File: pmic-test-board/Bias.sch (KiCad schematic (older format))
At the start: 19 parts, among them J301 Conn_Coaxial, J302 Conn_02x04_Odd_Even, U301 AZ431LANTR-G1, U302 DS4424N+

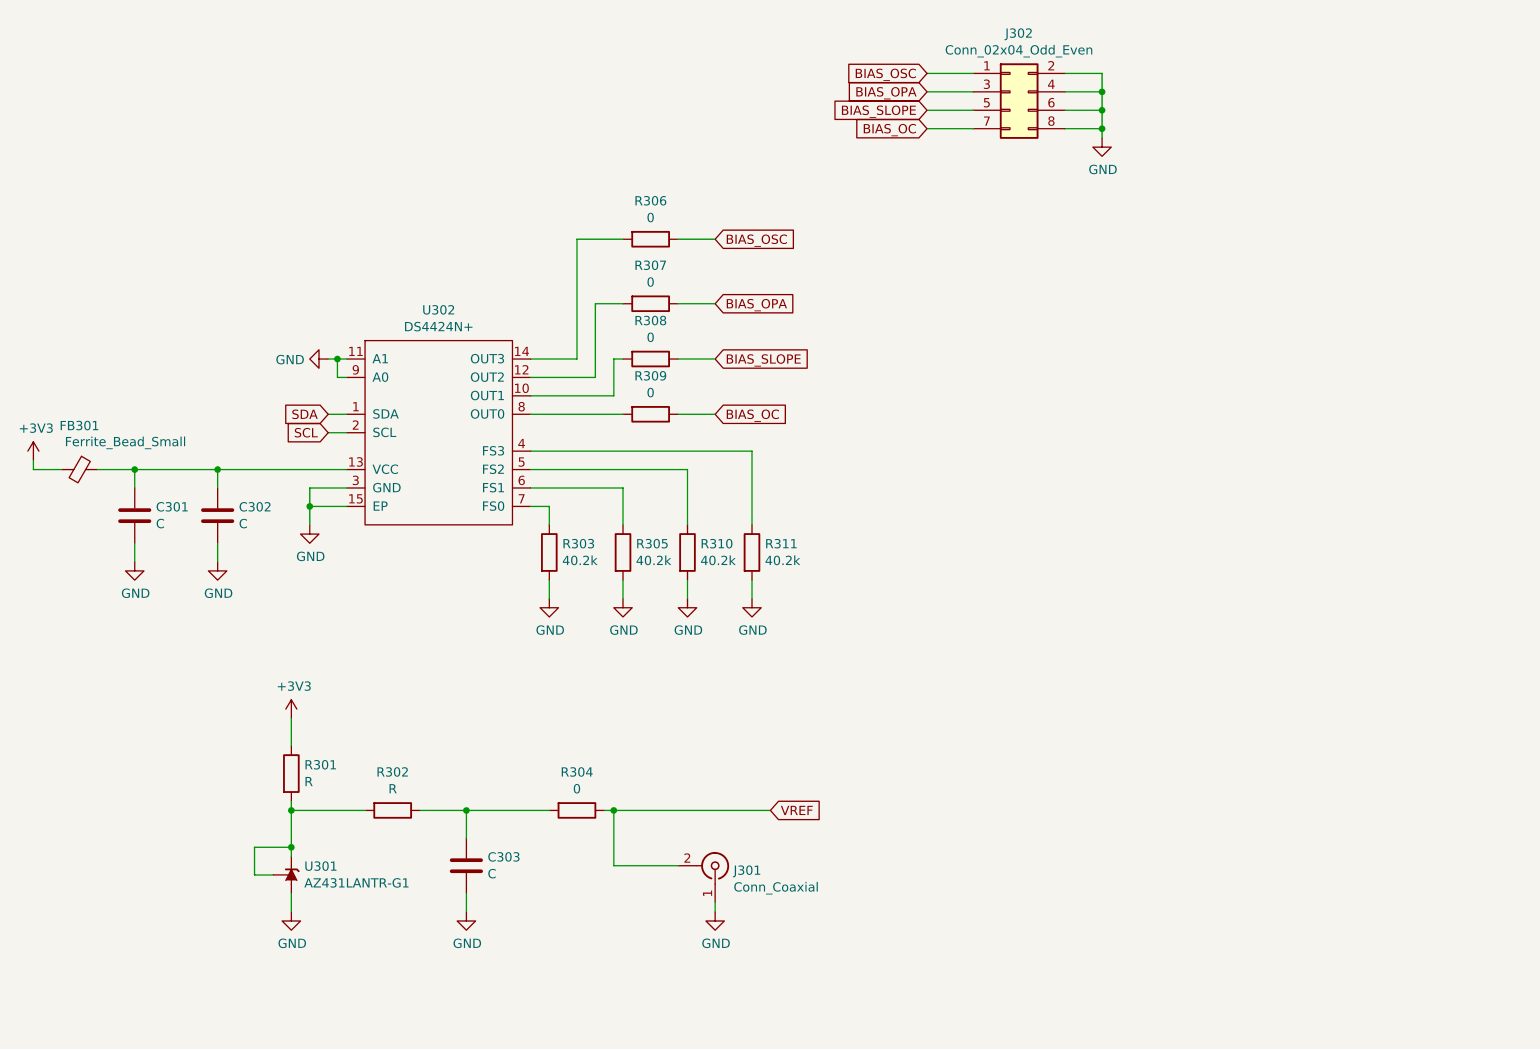
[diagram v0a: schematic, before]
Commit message: PCB routing done
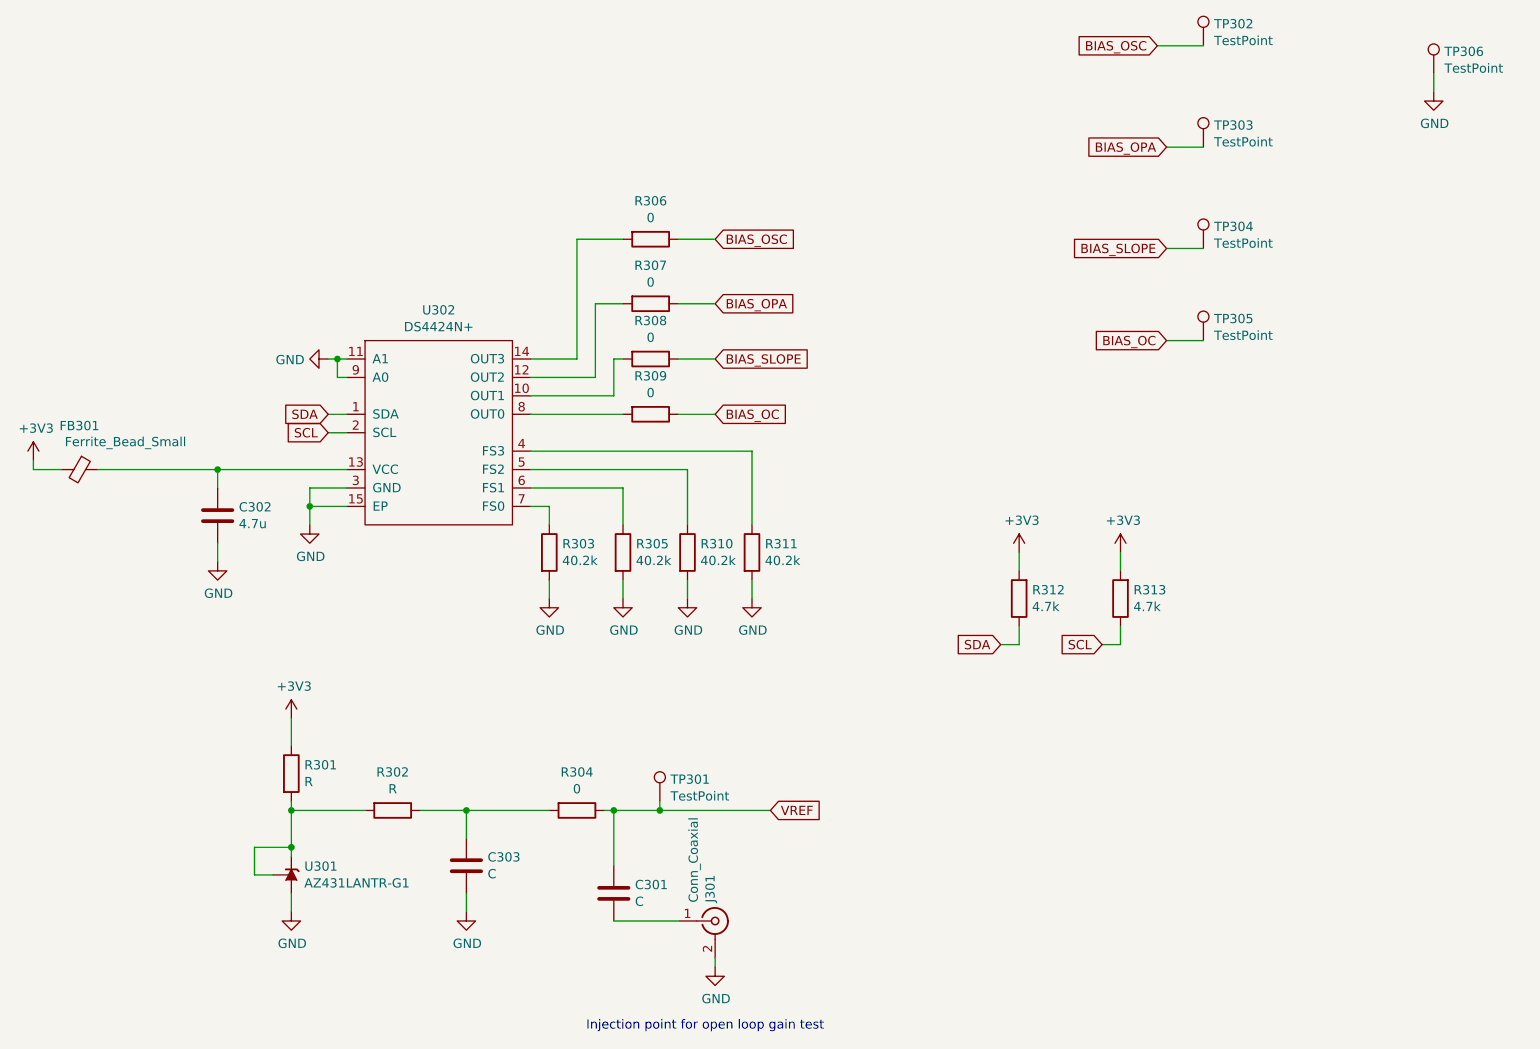
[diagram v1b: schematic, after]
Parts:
- removed J302: Conn_02x04_Odd_Even, symbol Connector_Generic:Conn_02x04_Odd_Even
- added R312, R313: 4.7k, Resistor_SMD:R_0603_1608Metric, symbol Device:R
- added TP301, TP302, TP303, TP304, TP305, TP306: TestPoint, wbraun_smd:THM_COMPACT, symbol Connector:TestPoint
- C302: value C -> 4.7u
- J301: footprint (none) -> Connector_Coaxial:SMA_Amphenol_132134_Vertical
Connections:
- net +3V3: now also R312.2, R313.2
- net BIAS_OC: now also TP305.1
- net BIAS_OPA: now also TP303.1
- net BIAS_OSC: now also TP302.1
- net BIAS_SLOPE: now also TP304.1
- net GND: now also J301.2 (Ext), TP306.1; no longer C301.2, J301.1 (In)
- net SCL: now also R313.1
- net SDA: now also R312.1
- net VREF: now also C301.1, TP301.1; no longer J301.2 (Ext)
- net at C302.1, FB301.1, U302.13 (VCC): no longer C301.1
- new net: C301.2, J301.1 (In)
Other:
- note added: "Injection point for open loop gain test"
- moved on the sheet: J301
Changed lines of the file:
@@
-$EndComp
-$Comp
-L Device:C C301
-U 1 1 619C3183
-P 1750 4100
-F 0 "C301" H 1865 4146 50  0000 L CNN
-F 1 "C" H 1865 4055 50  0000 L CNN
-F 2 "Capacitor_SMD:C_0603_1608Metric" H 1788 3950 50  0001 C CNN
-F 3 "~" H 1750 4100 50  0001 C CNN
-	1    1750 4100
-	1    0    0    -1
 $EndComp
 $Comp
@@
 P 2200 4100
 F 0 "C302" H 2315 4146 50  0000 L CNN
-F 1 "C" H 2315 4055 50  0000 L CNN
+F 1 "4.7u" H 2315 4055 50  0000 L CNN
 F 2 "Capacitor_SMD:C_0603_1608Metric" H 2238 3950 50  0001 C CNN
 F 3 "~" H 2200 4100 50  0001 C CNN
@@
 Wire Wire Line
 	2200 3950 2200 3850
-Wire Wire Line
-	1750 3950 1750 3850
-Wire Wire Line
-	1750 3850 2200 3850
-$Comp
-L power:GND #PWR0175
-U 1 1 619C47B0
-P 1750 4350
-F 0 "#PWR0175" H 1750 4100 50  0001 C CNN
-F 1 "GND" H 1755 4177 50  0000 C CNN
-F 2 "" H 1750 4350 50  0001 C CNN
-F 3 "" H 1750 4350 50  0001 C CNN
-	1    1750 4350
-	1    0    0    -1
-$EndComp
-Wire Wire Line
-	1750 4250 1750 4350
-Wire Wire Line
-	1550 3850 1750 3850
-Connection ~ 1750 3850
 Wire Wire Line
 	1350 3850 1200 3850
@@
 L Connector:Conn_Coaxial J301
 U 1 1 61A263C9
-P 4900 6000
-F 0 "J301" V 4874 6100 50  0000 L CNN
-F 1 "Conn_Coaxial" V 4783 6100 50  0000 L CNN
-F 2 "" H 4900 6000 50  0001 C CNN
-F 3 " ~" H 4900 6000 50  0001 C CNN
-	1    4900 6000
-	0    1    -1   0
+P 4900 6300
+F 0 "J301" V 4874 6400 50  0000 L CNN
+F 1 "Conn_Coaxial" V 4783 6400 50  0000 L CNN
+F 2 "Connector_Coaxial:SMA_Amphenol_132134_Vertical" H 4900 6300 50  0001 C CNN
+F 3 " ~" H 4900 6300 50  0001 C CNN
+	1    4900 6300
+	1    0    0    -1
 $EndComp
 $Comp
 L power:GND #PWR0185
 U 1 1 61A27901
-P 4900 6250
-F 0 "#PWR0185" H 4900 6000 50  0001 C CNN
-F 1 "GND" H 4905 6077 50  0000 C CNN
-F 2 "" H 4900 6250 50  0001 C CNN
-F 3 "" H 4900 6250 50  0001 C CNN
-	1    4900 6250
-	1    0    0    -1
-$EndComp
-Wire Wire Line
-	4900 6250 4900 6200
+P 4900 6550
+F 0 "#PWR0185" H 4900 6300 50  0001 C CNN
+F 1 "GND" H 4905 6377 50  0000 C CNN
+F 2 "" H 4900 6550 50  0001 C CNN
+F 3 "" H 4900 6550 50  0001 C CNN
+	1    4900 6550
+	1    0    0    -1
+$EndComp
+Wire Wire Line
+	4900 6550 4900 6500
 $Comp
 L Device:R R304
@@
 $EndComp
 Wire Wire Line
-	4700 6000 4350 6000
+	4700 6300 4350 6300
 Wire Wire Line
 	4350 6000 4350 5700
@@
 	4350 5700 4300 5700
 Wire Wire Line
-	4350 5700 5200 5700
+	4350 5700 4600 5700
 Connection ~ 4350 5700
 Text GLabel 5200 5700 2    50   Input ~ 0
 VREF
-$Comp
-L Connector_Generic:Conn_02x04_Odd_Even J302
-U 1 1 61A2AA7E
-P 6500 1800
-F 0 "J302" H 6550 2117 50  0000 C CNN
-F 1 "Conn_02x04_Odd_Even" H 6550 2026 50  0000 C CNN
-F 2 "" H 6500 1800 50  0001 C CNN
-F 3 "~" H 6500 1800 50  0001 C CNN
-	1    6500 1800
-	1    0    0    -1
-$EndComp
 $Comp
 L Device:R R306
@@
 Text GLabel 4900 3550 2    50   Input ~ 0
 BIAS_OC
-$Comp
-L power:GND #PWR0186
-U 1 1 61A39A05
-P 7000 2050
-F 0 "#PWR0186" H 7000 1800 50  0001 C CNN
-F 1 "GND" H 7005 1877 50  0000 C CNN
-F 2 "" H 7000 2050 50  0001 C CNN
-F 3 "" H 7000 2050 50  0001 C CNN
-	1    7000 2050
-	1    0    0    -1
-$EndComp
-Text GLabel 6050 1700 0    50   Input ~ 0
+Text GLabel 7300 1550 0    50   Input ~ 0
 BIAS_OSC
-Text GLabel 6050 1800 0    50   Input ~ 0
+Text GLabel 7350 2100 0    50   Input ~ 0
 BIAS_OPA
-Text GLabel 6050 1900 0    50   Input ~ 0
+Text GLabel 7350 2650 0    50   Input ~ 0
 BIAS_SLOPE
-Text GLabel 6050 2000 0    50   Input ~ 0
+Text GLabel 7350 3150 0    50   Input ~ 0
 BIAS_OC
-Wire Wire Line
-	6300 1700 6050 1700
-Wire Wire Line
-	6300 1800 6050 1800
-Wire Wire Line
-	6300 1900 6050 1900
-Wire Wire Line
-	6300 2000 6050 2000
-Wire Wire Line
-	6800 1700 7000 1700
-Wire Wire Line
-	7000 1700 7000 1800
-Wire Wire Line
-	6800 1800 7000 1800
-Connection ~ 7000 1800
-Wire Wire Line
-	7000 1800 7000 1900
-Wire Wire Line
-	6800 1900 7000 1900
-Connection ~ 7000 1900
-Wire Wire Line
-	7000 1900 7000 2000
-Wire Wire Line
-	6800 2000 7000 2000
-Connection ~ 7000 2000
-Wire Wire Line
-	7000 2000 7000 2050
+$Comp
+L Connector:TestPoint TP302
+U 1 1 6219CA5D
+P 7550 1550
+F 0 "TP302" H 7608 1668 50  0000 L CNN
+F 1 "TestPoint" H 7608 1577 50  0000 L CNN
+F 2 "wbraun_smd:THM_COMPACT" H 7750 1550 50  0001 C CNN
+F 3 "~" H 7750 1550 50  0001 C CNN
+	1    7550 1550
+	1    0    0    -1
+$EndComp
+$Comp
+L Connector:TestPoint TP303
+U 1 1 6219E164
+P 7550 2100
+F 0 "TP303" H 7608 2218 50  0000 L CNN
+F 1 "TestPoint" H 7608 2127 50  0000 L CNN
+F 2 "wbraun_smd:THM_COMPACT" H 7750 2100 50  0001 C CNN
+F 3 "~" H 7750 2100 50  0001 C CNN
+	1    7550 2100
+	1    0    0    -1
+$EndComp
+$Comp
+L Connector:TestPoint TP304
+U 1 1 6219E716
+P 7550 2650
+F 0 "TP304" H 7608 2768 50  0000 L CNN
+F 1 "TestPoint" H 7608 2677 50  0000 L CNN
+F 2 "wbraun_smd:THM_COMPACT" H 7750 2650 50  0001 C CNN
+F 3 "~" H 7750 2650 50  0001 C CNN
+	1    7550 2650
+	1    0    0    -1
+$EndComp
+$Comp
+L Connector:TestPoint TP305
+U 1 1 6219EA0B
+P 7550 3150
+F 0 "TP305" H 7608 3268 50  0000 L CNN
+F 1 "TestPoint" H 7608 3177 50  0000 L CNN
+F 2 "wbraun_smd:THM_COMPACT" H 7750 3150 50  0001 C CNN
+F 3 "~" H 7750 3150 50  0001 C CNN
+	1    7550 3150
+	1    0    0    -1
+$EndComp
+Wire Wire Line
+	7350 3150 7550 3150
+Wire Wire Line
+	7350 2650 7550 2650
+Wire Wire Line
+	7350 2100 7550 2100
+Wire Wire Line
+	7300 1550 7550 1550
+$Comp
+L power:GND #PWR0237
+U 1 1 621A3B1A
+P 8800 1800
+F 0 "#PWR0237" H 8800 1550 50  0001 C CNN
+F 1 "GND" H 8805 1627 50  0000 C CNN
+F 2 "" H 8800 1800 50  0001 C CNN
+F 3 "" H 8800 1800 50  0001 C CNN
+	1    8800 1800
+	1    0    0    -1
+$EndComp
+$Comp
+L Connector:TestPoint TP306
+U 1 1 621A3EC4
+P 8800 1700
+F 0 "TP306" H 8858 1818 50  0000 L CNN
+F 1 "TestPoint" H 8858 1727 50  0000 L CNN
+F 2 "wbraun_smd:THM_COMPACT" H 9000 1700 50  0001 C CNN
+F 3 "~" H 9000 1700 50  0001 C CNN
+	1    8800 1700
+	1    0    0    -1
+$EndComp
+Wire Wire Line
+	8800 1700 8800 1800
+$Comp
+L Connector:TestPoint TP301
+U 1 1 62459C59
+P 4600 5650
+F 0 "TP301" H 4658 5768 50  0000 L CNN
+F 1 "TestPoint" H 4658 5677 50  0000 L CNN
+F 2 "wbraun_smd:THM_COMPACT" H 4800 5650 50  0001 C CNN
+F 3 "~" H 4800 5650 50  0001 C CNN
+	1    4600 5650
+	1    0    0    -1
+$EndComp
+Wire Wire Line
+	4600 5650 4600 5700
+Connection ~ 4600 5700
+Wire Wire Line
+	4600 5700 5200 5700
+Wire Wire Line
+	1550 3850 2200 3850
+$Comp
+L Device:C C301
+U 1 1 62A9AC31
+P 4350 6150
+F 0 "C301" H 4465 6196 50  0000 L CNN
+F 1 "C" H 4465 6105 50  0000 L CNN
+F 2 "Capacitor_SMD:C_0603_1608Metric" H 4388 6000 50  0001 C CNN
+F 3 "~" H 4350 6150 50  0001 C CNN
+	1    4350 6150
+	1    0    0    -1
+$EndComp
+Text Notes 4200 6900 0    50   ~ 0
+Injection point for open loop gain test
+$Comp
+L Device:R R?
+U 1 1 61E477C4
+P 6550 4550
+AR Path="/61E477C4" Ref="R?"  Part="1"
+AR Path="/61997357/61E477C4" Ref="R312"  Part="1"
+F 0 "R312" H 6480 4504 50  0000 R CNN
+F 1 "4.7k" H 6480 4595 50  0000 R CNN
+F 2 "Resistor_SMD:R_0603_1608Metric" V 6480 4550 50  0001 C CNN
+F 3 "~" H 6550 4550 50  0001 C CNN
+	1    6550 4550
+	-1   0    0    1
+$EndComp
+$Comp
+L power:+3V3 #PWR0168
+U 1 1 61E4A9AD
+P 6550 4300
+F 0 "#PWR0168" H 6550 4150 50  0001 C CNN
+F 1 "+3V3" H 6565 4473 50  0000 C CNN
+F 2 "" H 6550 4300 50  0001 C CNN
+F 3 "" H 6550 4300 50  0001 C CNN
+	1    6550 4300
+	1    0    0    -1
+$EndComp
+Text GLabel 6450 4800 0    50   Input ~ 0
+SDA
+Wire Wire Line
+	6550 4300 6550 4400
+Wire Wire Line
+	6450 4800 6550 4800
+Wire Wire Line
+	6550 4700 6550 4800
+$Comp
+L Device:R R?
+U 1 1 61E5127E
+P 7100 4550
+AR Path="/61E5127E" Ref="R?"  Part="1"
+AR Path="/61997357/61E5127E" Ref="R313"  Part="1"
+F 0 "R313" H 7030 4504 50  0000 R CNN
+F 1 "4.7k" H 7030 4595 50  0000 R CNN
+F 2 "Resistor_SMD:R_0603_1608Metric" V 7030 4550 50  0001 C CNN
+F 3 "~" H 7100 4550 50  0001 C CNN
+	1    7100 4550
+	-1   0    0    1
+$EndComp
+$Comp
+L power:+3V3 #PWR0169
+U 1 1 61E51284
+P 7100 4300
+F 0 "#PWR0169" H 7100 4150 50  0001 C CNN
+F 1 "+3V3" H 7115 4473 50  0000 C CNN
+F 2 "" H 7100 4300 50  0001 C CNN
+F 3 "" H 7100 4300 50  0001 C CNN
+	1    7100 4300
+	1    0    0    -1
+$EndComp
+Wire Wire Line
+	7100 4300 7100 4400
+Wire Wire Line
+	7100 4700 7100 4800
+Text GLabel 7000 4800 0    50   Input ~ 0
+SCL
+Wire Wire Line
+	7000 4800 7100 4800
 $EndSCHEMATC
